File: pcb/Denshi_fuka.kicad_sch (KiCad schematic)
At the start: 21 parts, among them J1 Power, J2 Digital/PWM, J3 Analog, J4 Digital/PWM, Q1 NMOS, Q2 NMOS, U1 LM358, U3 ADS1115IDGS, U4 MCP6002-xP, U5 MCP4728, U6 ISO1540

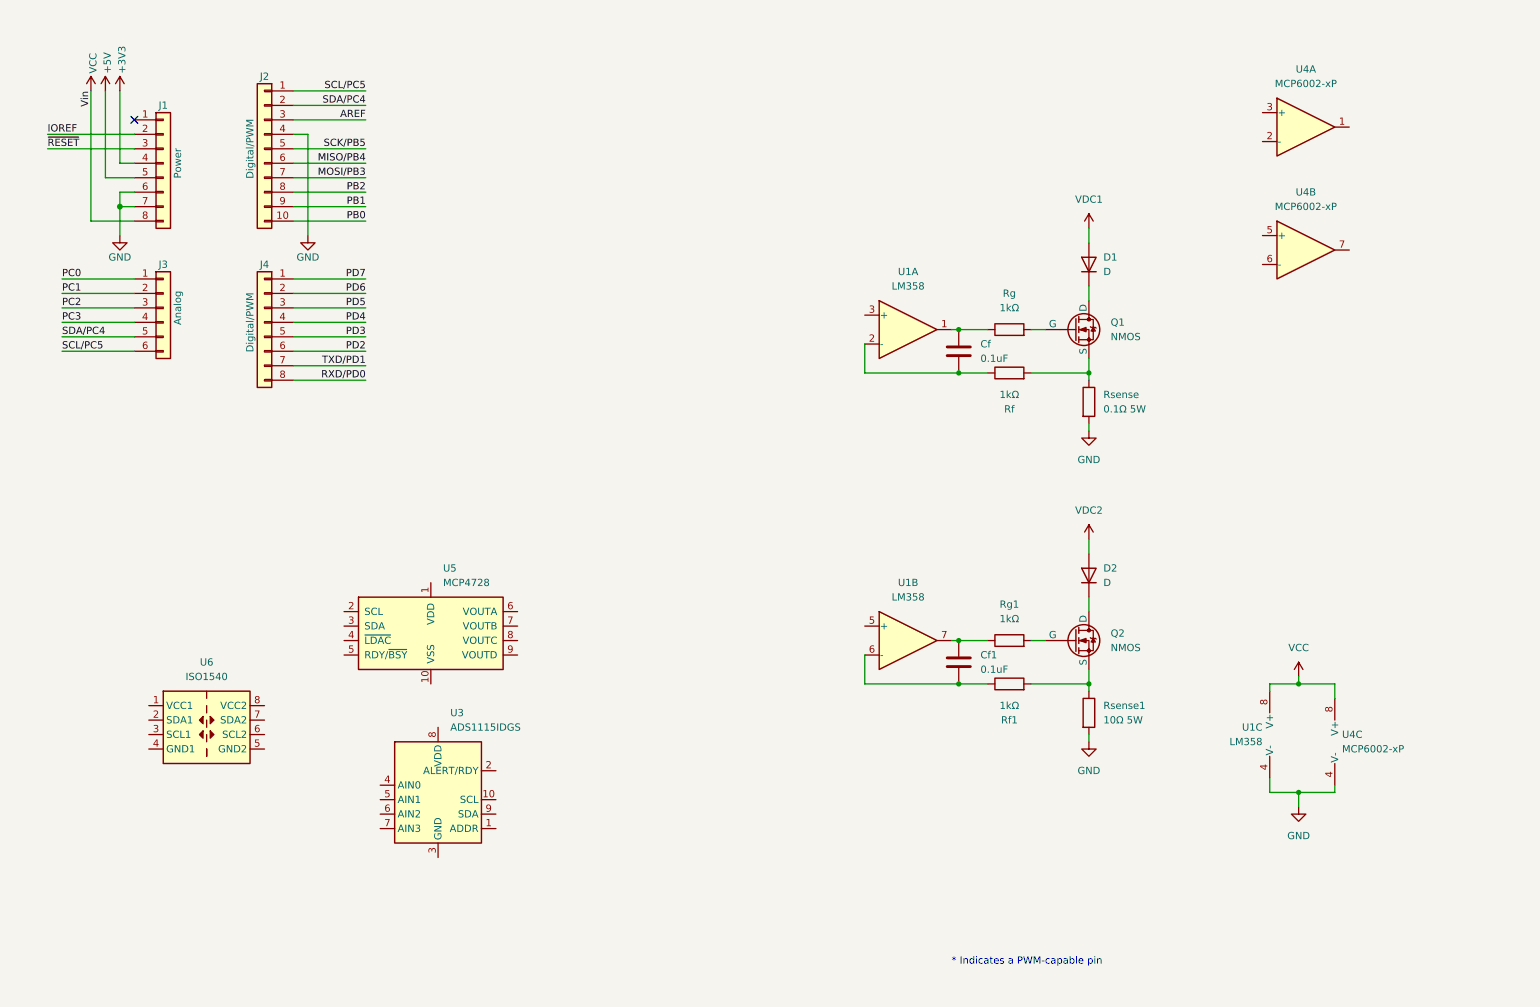
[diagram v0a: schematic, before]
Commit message: schematic completed!
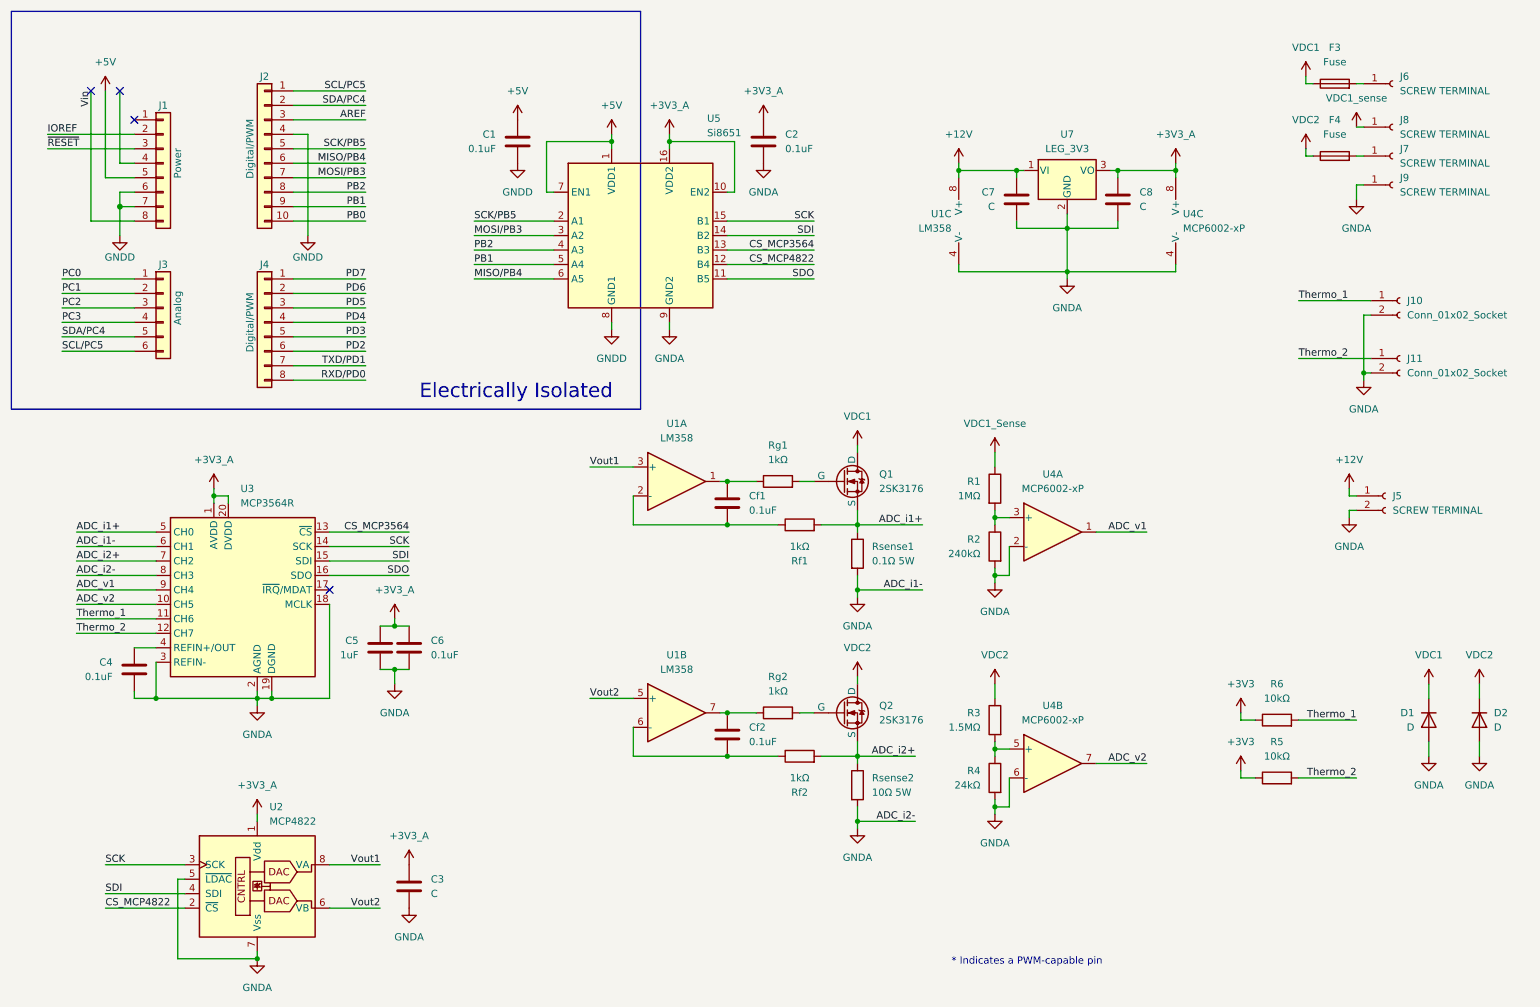
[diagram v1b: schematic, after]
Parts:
- removed U3: ADS1115IDGS, Package_SO:TSSOP-10_3x3mm_P0.5mm, symbol Analog_ADC:ADS1115IDGS
- removed U5: MCP4728, Package_SO:MSOP-10_3x3mm_P0.5mm, symbol Analog_DAC:MCP4728
- removed U6: ISO1540, Package_SO:SOIC-8_3.9x4.9mm_P1.27mm, symbol Isolator:ISO1540
- added C1, C2, C4, C6: 0.1uF, Capacitor_THT:C_Disc_D5.0mm_W2.5mm_P5.00mm, symbol Device:C
- added C3, C7, C8: C, symbol Device:C
- added C5: 1uF, Capacitor_THT:C_Disc_D5.0mm_W2.5mm_P5.00mm, symbol Device:C
- added F3, F4: Fuse, symbol Device:Fuse
- added J10, J11: Conn_01x02_Socket, symbol Connector:Conn_01x02_Socket
- added J5: SCREW TERMINAL, symbol Connector:Conn_01x02_Socket
- added J6, J7, J8, J9: SCREW TERMINAL, symbol Connector:Conn_01x01_Socket
- added R1: 1MΩ, Resistor_THT:R_Axial_DIN0207_L6.3mm_D2.5mm_P10.16mm_Horizontal, symbol Device:R
- added R2: 240kΩ, Resistor_THT:R_Axial_DIN0207_L6.3mm_D2.5mm_P10.16mm_Horizontal, symbol Device:R
- added R3: 1.5MΩ, Resistor_THT:R_Axial_DIN0207_L6.3mm_D2.5mm_P10.16mm_Horizontal, symbol Device:R
- added R4: 24kΩ, Resistor_THT:R_Axial_DIN0207_L6.3mm_D2.5mm_P10.16mm_Horizontal, symbol Device:R
- added R5, R6: 10kΩ, symbol Device:R
- added U2: MCP4822, Package_DIP:DIP-8_W7.62mm_Socket_LongPads, symbol Analog_DAC:MCP4822
- added U3: MCP3564R, symbol Fuka_sym:MCP3564R
- added U5: Si8651, symbol Fuka_sym:Si8651
- added U7: LEG_3V3, Package_TO_SOT_THT:TO-220-3_Vertical, symbol Regulator_Linear:LM7805_TO220
- Cf1: renamed from Cf; footprint (none) -> Capacitor_THT:C_Disc_D5.0mm_W2.5mm_P5.00mm
- Cf2: renamed from Cf1; footprint (none) -> Capacitor_THT:C_Disc_D5.0mm_W2.5mm_P5.00mm
- D1, D2: footprint (none) -> Package_TO_SOT_THT:TO-220-2_Vertical
- Q1, Q2: value NMOS -> 2SK3176; footprint (none) -> Package_TO_SOT_THT:TO-247-3_Horizontal_TabUp
- Rf1: renamed from Rf; footprint (none) -> Resistor_THT:R_Axial_DIN0207_L6.3mm_D2.5mm_P10.16mm_Horizontal
- Rf2: renamed from Rf1; footprint (none) -> Resistor_THT:R_Axial_DIN0207_L6.3mm_D2.5mm_P10.16mm_Horizontal
- Rg1: renamed from Rg; footprint (none) -> Resistor_THT:R_Axial_DIN0207_L6.3mm_D2.5mm_P10.16mm_Horizontal
- Rg2: renamed from Rg1; footprint (none) -> Resistor_THT:R_Axial_DIN0207_L6.3mm_D2.5mm_P10.16mm_Horizontal
- Rsense1: renamed from Rsense; footprint (none) -> Resistor_THT:R_Axial_Power_L48.0mm_W12.5mm_P55.88mm
- Rsense2: renamed from Rsense1; footprint (none) -> Resistor_THT:R_Axial_Power_L48.0mm_W12.5mm_P55.88mm
- U4: footprint (none) -> Package_DIP:DIP-8_W7.62mm_Socket_LongPads
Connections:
- net +3V3: now also R5.1, R6.1; no longer J1.4 (Pin_4)
- net +5V: now also C1.1, U5.1 (VDD1), U5.7 (EN1)
- net MISO/PB4: now also U5.6 (A5)
- net MOSI/PB3: now also U5.3 (A2)
- net PB1: now also U5.5 (A4)
- net PB2: now also U5.4 (A3)
- net SCK/PB5: now also U5.2 (A1)
- net VDC1: now also D1.1 (K), Q1.1 (D), F3.1; no longer D1.2 (A)
- net VDC2: now also D2.1 (K), Q2.1 (D), F4.1, R3.1; no longer D2.2 (A)
- net ADC_i2+: now reaches Q2.3 (S), Rf2.2, Rsense2.1
- net ADC_i2+: now also U3.7 (CH2)
- net ADC_i1+: now reaches Q1.3 (S), Rf1.2, Rsense1.1
- net ADC_i1+: now also U3.5 (CH0)
- net at U4.5 (+): now also R3.2, R4.1
- net GNDA: now reaches U4.6 (-)
- net GNDA: now also D1.2 (A), D2.2 (A), Rsense1.2, Rsense2.2, U1.4 (V-), U4.2 (-), U4.4 (V-), C2.2, C3.2, C4.2, C5.2, C6.2, C7.2, C8.2, J10.2 (Pin_2), J11.2 (Pin_2), J5.2 (Pin_2), J9.1 (Pin_1), R2.2, R4.2, U2.5 (~{LDAC}), U2.7 (Vss), U3.18 (MCLK), U3.19 (DGND), U3.2 (AGND), U3.3 (REFIN-), U3.6 (CH1), U3.8 (CH3), U5.9 (GND2), U7.2 (GND)
- net ADC_v2: now reaches U4.7
- net ADC_v2: now also U3.10 (CH5)
- net Vout1: now reaches U1.3 (+)
- net Vout1: now also U2.8 (VA)
- net Vout2: now reaches U1.5 (+)
- net Vout2: now also U2.6 (VB)
- net ADC_v1: now reaches U4.1
- net ADC_v1: now also U3.9 (CH4)
- net at U4.3 (+): now also R1.2, R2.1
- removed net GND: J1.6 (Pin_6), J1.7 (Pin_7), J2.4 (Pin_4), Rsense1.2, Rsense2.2, U1.4 (V-), U4.4 (V-)
- removed net VCC: J1.8 (Pin_8), U1.8 (V+), U4.8 (V+)
- new net: F4.2, J7.1 (Pin_1)
- new net: F3.2, J6.1 (Pin_1)
- new net: C4.1, U3.4 (REFIN+/OUT)
- new net +12V: C7.1, J5.1 (Pin_1), U1.8 (V+), U7.1 (VI)
- new net +3V3_A: C2.1, C3.1, C5.1, C6.1, C8.1, U2.1 (Vdd), U3.1 (AVDD), U3.20 (DVDD), U4.8 (V+), U5.10 (EN2), U5.16 (VDD2), U7.3 (VO)
- new net CS_MCP3564: U3.13 (~{CS}), U5.13 (B3)
- new net CS_MCP4822: U2.2 (~{CS}), U5.12 (B4)
- new net GNDD: C1.2, J1.6 (Pin_6), J1.7 (Pin_7), J2.4 (Pin_4), U5.8 (GND1)
- new net SCK: U2.3 (SCK), U3.14 (SCK), U5.15 (B1)
- new net SDI: U2.4 (SDI), U3.15 (SDI), U5.14 (B2)
- new net SDO: U3.16 (SDO), U5.11 (B5)
- new net Thermo_1: J10.1 (Pin_1), R6.2, U3.11 (CH6)
- new net Thermo_2: J11.1 (Pin_1), R5.2, U3.12 (CH7)
- new net VDC1_Sense: R1.1
- new net VDC1_sense: J8.1 (Pin_1)
- new net Vin: J1.8 (Pin_8)
- no-connect marks 1 -> 4
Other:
- note added: "Electrically Isolated"
- moved on the sheet: Cf1, Cf2, Q1, Q2, Rf1, Rf2, Rg1, Rg2, Rsense1, Rsense2, U1A, U1B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
